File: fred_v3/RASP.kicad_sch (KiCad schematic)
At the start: 18 parts, among them J12 Conn_02x20_Odd_Even, J13 FAN1, J14 FAN2, J15 FAN3, J16 FAN4, Q7 NMOS, U14 MCP2515-xSO, Y1 Crystal

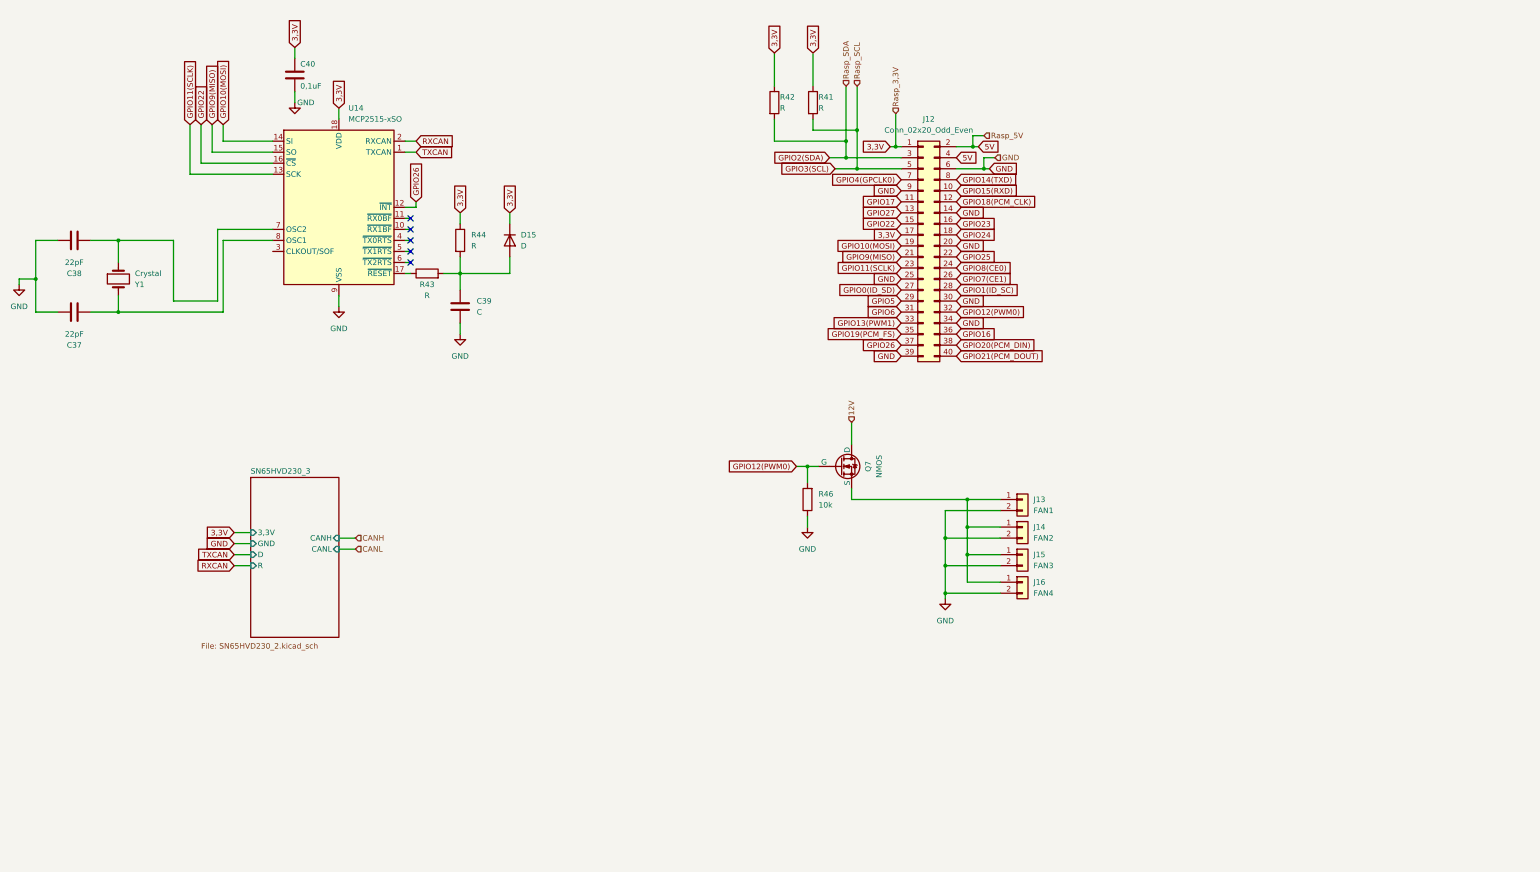
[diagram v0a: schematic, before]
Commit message: Add files via upload
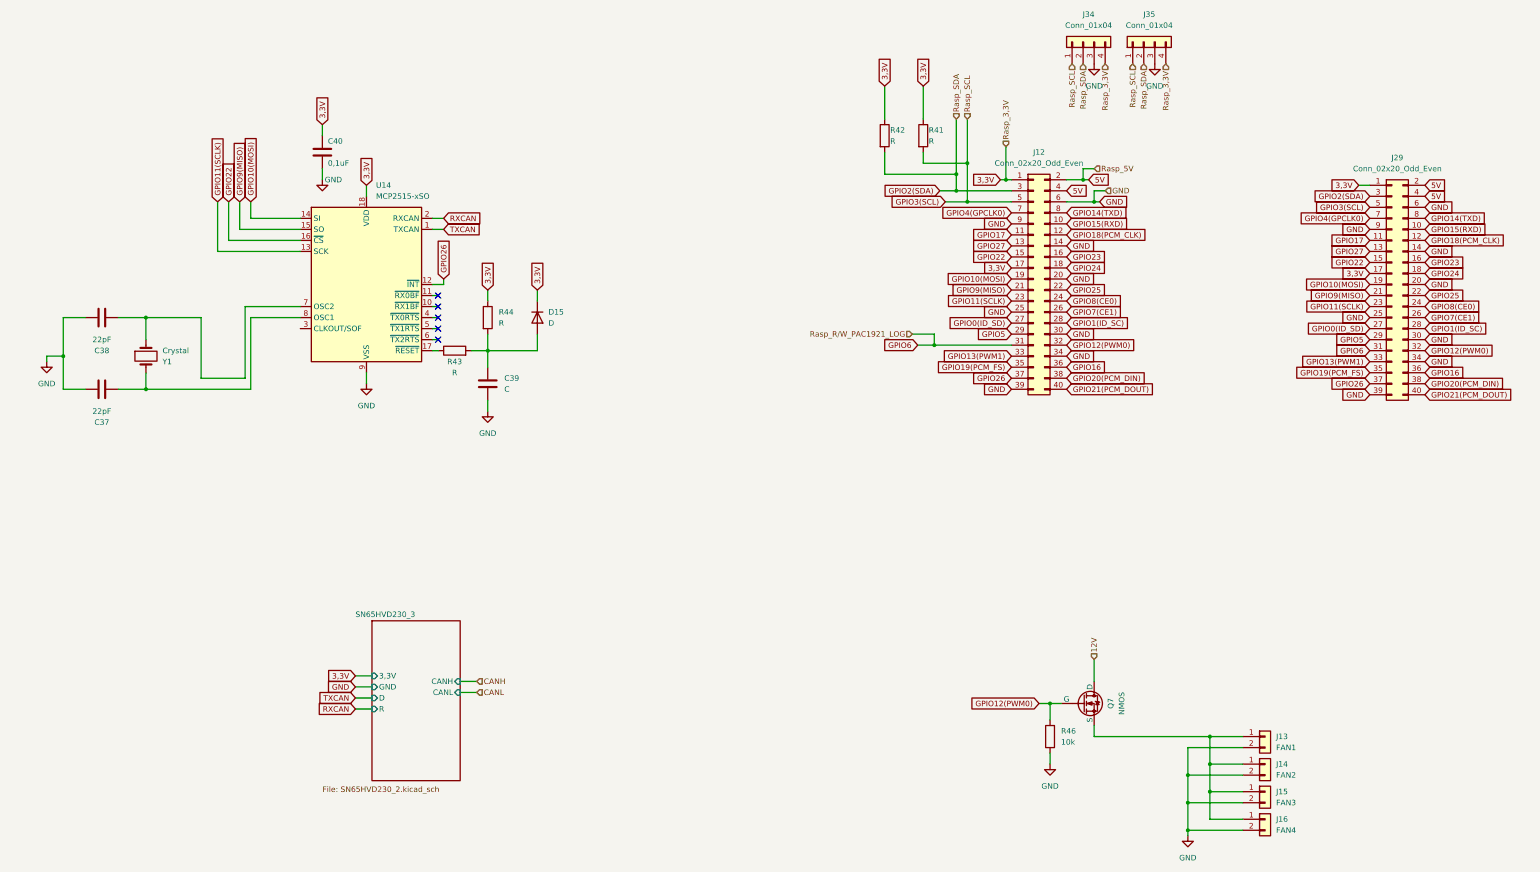
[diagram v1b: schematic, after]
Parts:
- added J29: Conn_02x20_Odd_Even, Connector_PinSocket_2.54mm:PinSocket_2x20_P2.54mm_Vertical, symbol Connector_Generic:Conn_02x20_Odd_Even
- added J34, J35: Conn_01x04, Connector_JST:JST_EH_S4B-EH_1x04_P2.50mm_Horizontal, symbol Connector_Generic:Conn_01x04
- C37, C38, C39, C40: footprint (none) -> Capacitor_SMD:C_0603_1608Metric_Pad1.08x0.95mm_HandSolder
- D15: footprint (none) -> Diode_SMD:D_SOD-128
- J12: footprint (none) -> Connector_PinSocket_2.54mm:PinSocket_2x20_P2.54mm_Vertical
- J13, J14, J15, J16: footprint (none) -> Connector_JST:JST_EH_B2B-EH-A_1x02_P2.50mm_Vertical
- Q7: footprint (none) -> Package_TO_SOT_SMD:TO-252-2
- R41, R42, R43, R44, R46: footprint (none) -> Resistor_SMD:R_0603_1608Metric_Pad0.98x0.95mm_HandSolder
- Y1: footprint (none) -> Crystal:Crystal_HC49-4H_Vertical
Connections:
- net 3,3V: now also J29.1 (Pin_1), J29.17 (Pin_17), J34.4 (Pin_4), J35.4 (Pin_4)
- net 5V: now also J29.2 (Pin_2), J29.4 (Pin_4)
- net GND: now also J29.14 (Pin_14), J29.20 (Pin_20), J29.25 (Pin_25), J29.30 (Pin_30), J29.34 (Pin_34), J29.39 (Pin_39), J29.6 (Pin_6), J29.9 (Pin_9), J34.3 (Pin_3), J35.3 (Pin_3)
- net GPIO0(ID_SD): now also J29.27 (Pin_27)
- net GPIO1(ID_SC): now also J29.28 (Pin_28)
- net GPIO10(MOSI): now also J29.19 (Pin_19)
- net GPIO11(SCLK): now also J29.23 (Pin_23)
- net GPIO12(PWM0): now also J29.32 (Pin_32)
- net GPIO13(PWM1): now also J29.33 (Pin_33)
- net GPIO14(TXD): now also J29.8 (Pin_8)
- net GPIO15(RXD): now also J29.10 (Pin_10)
- net GPIO16: now also J29.36 (Pin_36)
- net GPIO17: now also J29.11 (Pin_11)
- net GPIO18(PCM_CLK): now also J29.12 (Pin_12)
- net GPIO19(PCM_FS): now also J29.35 (Pin_35)
- net GPIO2(SDA): now also J29.3 (Pin_3), J34.2 (Pin_2), J35.2 (Pin_2)
- net GPIO20(PCM_DIN): now also J29.38 (Pin_38)
- net GPIO21(PCM_DOUT): now also J29.40 (Pin_40)
- net GPIO22: now also J29.15 (Pin_15)
- net GPIO23: now also J29.16 (Pin_16)
- net GPIO24: now also J29.18 (Pin_18)
- net GPIO25: now also J29.22 (Pin_22)
- net GPIO26: now also J29.37 (Pin_37)
- net GPIO27: now also J29.13 (Pin_13)
- net GPIO3(SCL): now also J29.5 (Pin_5), J34.1 (Pin_1), J35.1 (Pin_1)
- net GPIO4(GPCLK0): now also J29.7 (Pin_7)
- net GPIO5: now also J29.29 (Pin_29)
- net GPIO6: now also J29.31 (Pin_31)
- net GPIO7(CE1): now also J29.26 (Pin_26)
- net GPIO8(CE0): now also J29.24 (Pin_24)
- net GPIO9(MISO): now also J29.21 (Pin_21)
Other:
- moved on the sheet: C37, C38, C39, C40, D15, J12, J13, J14, J15, J16, Q7, R41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
